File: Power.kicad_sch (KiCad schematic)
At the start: 11 parts, among them U3 TPS2121RUXR, U4 TPS62152RGTR

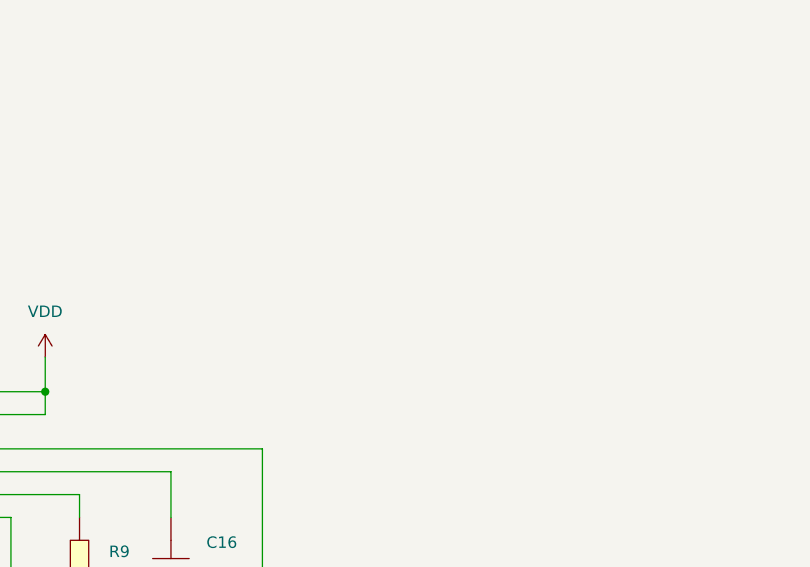
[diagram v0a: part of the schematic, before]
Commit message: switched to RP2350A and added flash chip due to parts shortage
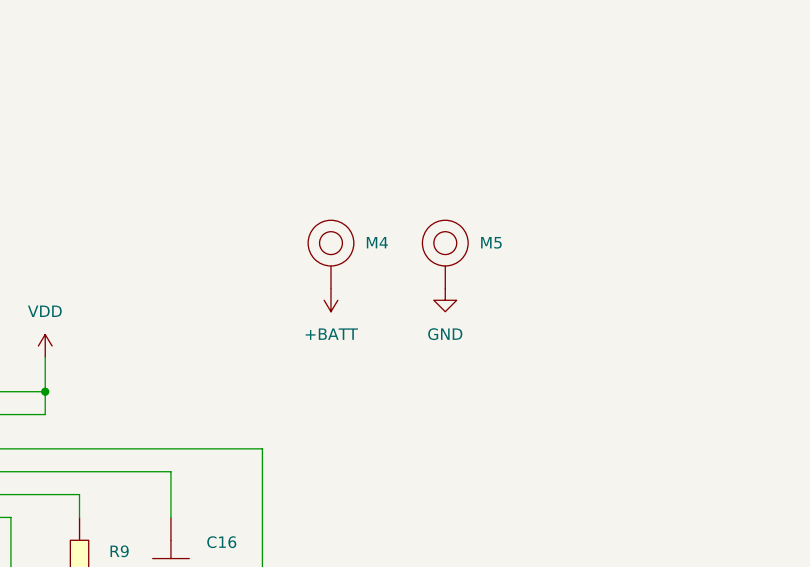
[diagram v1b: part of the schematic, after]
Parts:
- added M4, M5: (no value), Other:M2_Hole, symbol Other:M2_Hole
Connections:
- net +BATT: now also M4. (1)
- net GND: now also M5. (1)

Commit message: Final manufactured version
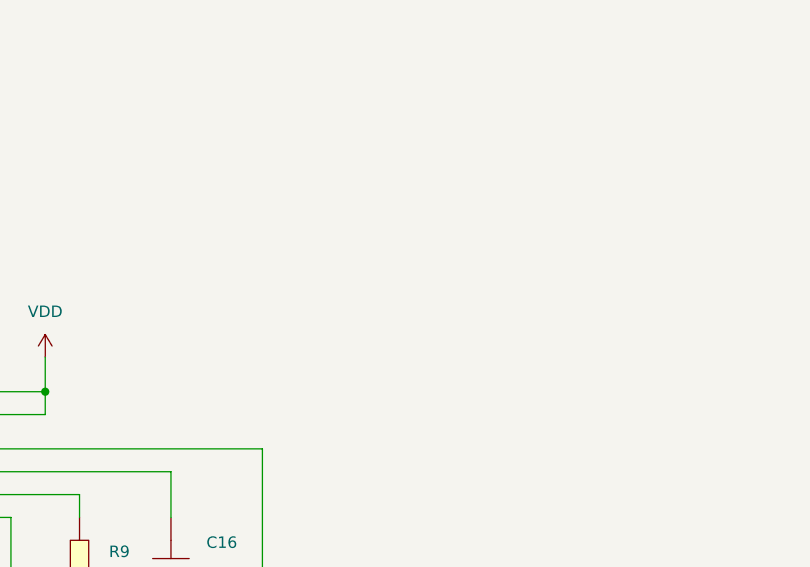
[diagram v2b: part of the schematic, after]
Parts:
- removed M4, M5: (no value), Other:M2_Hole, symbol Other:M2_Hole
